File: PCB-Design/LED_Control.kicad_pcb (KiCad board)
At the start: 2 copper layers, 60 x 80 mm, 28 parts, among them J1 5V 5A Power, J2 TO WS2812B LED STRIP, J3 Sound Sensor, SW1 SW_Push_Dual

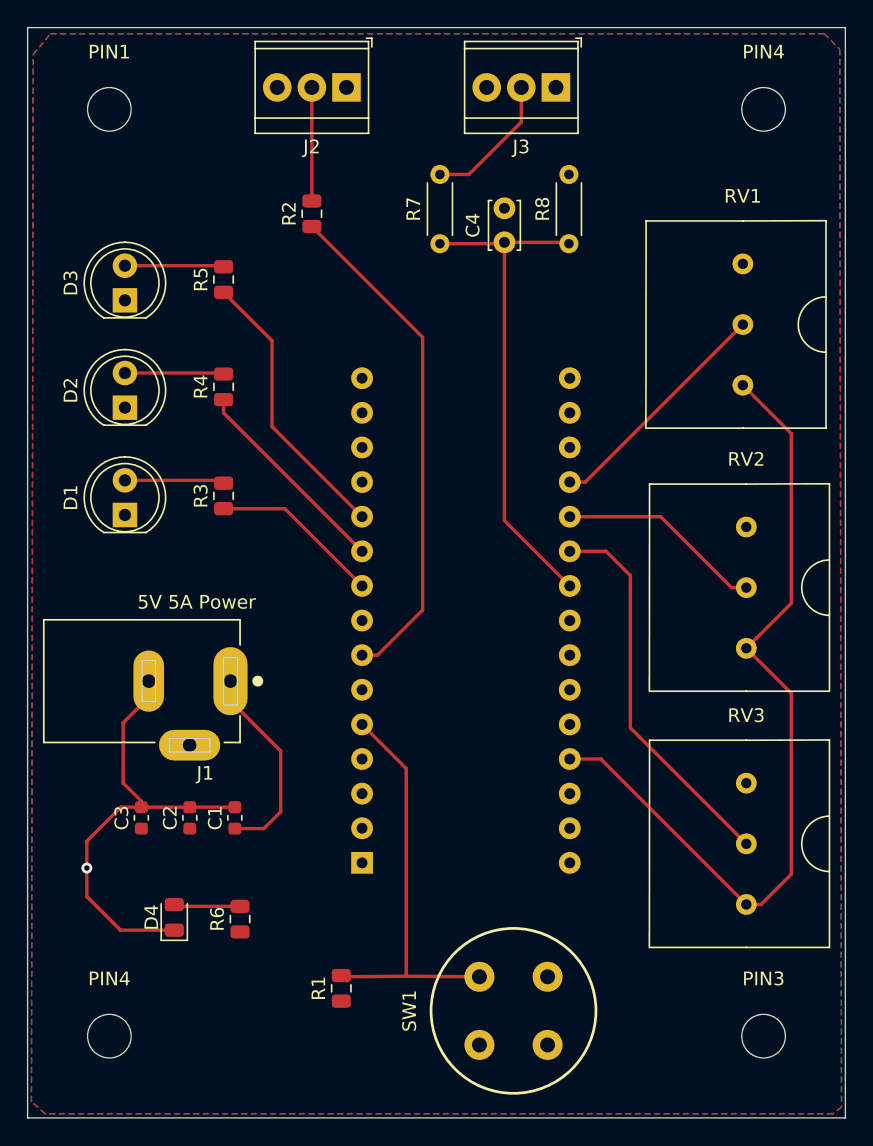
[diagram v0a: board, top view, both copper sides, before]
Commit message: final submitted build files
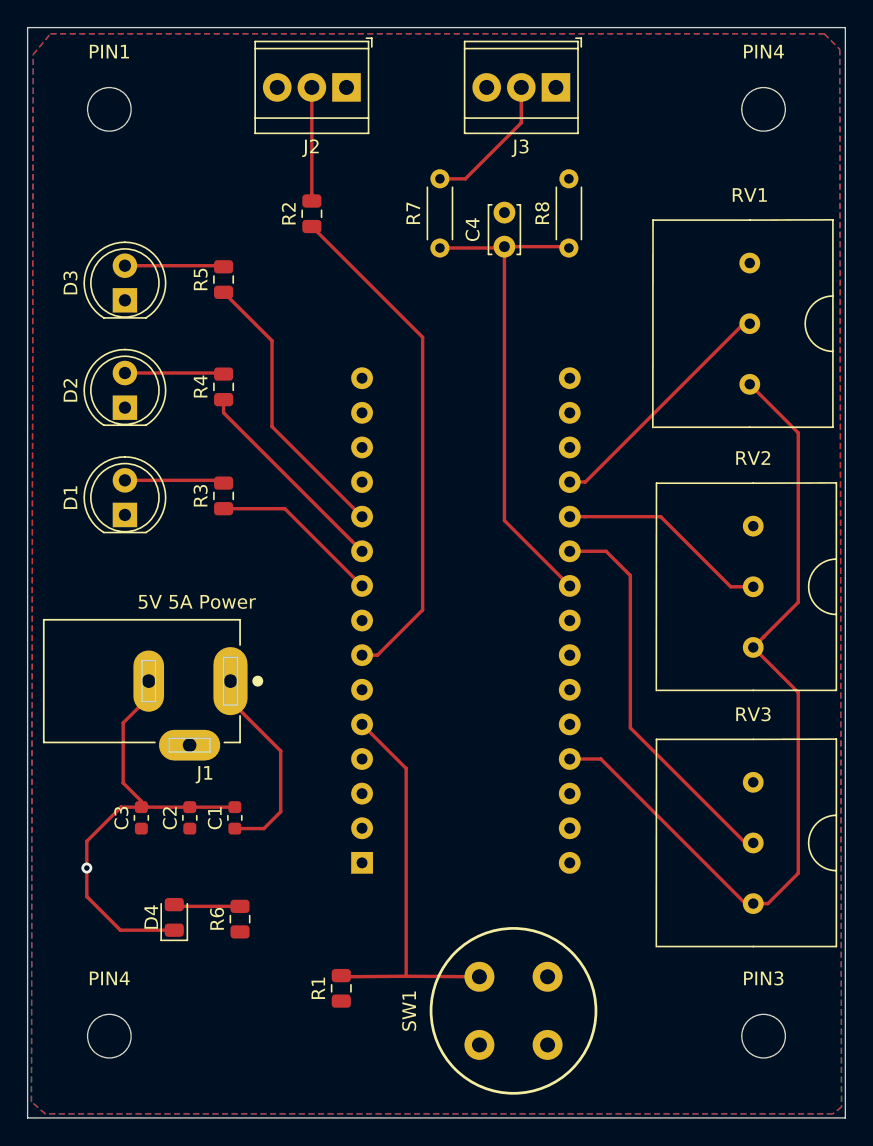
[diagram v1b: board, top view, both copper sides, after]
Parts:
- R6: value 100 -> 200
- moved RV1 0.51 mm to (158.0, 81.7)
- moved RV2 0.51 mm to (158.2, 101.0)
- moved RV3 0.51 mm to (158.2, 119.8)
- moved C4 0.32 mm to (140.0, 76.1)
- moved R7 0.32 mm to (135.3, 76.2)
- moved R8 0.32 mm to (144.7, 76.2)
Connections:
- J3 pad 1: GND -> VCC
- J3 pad 3: VCC -> GND
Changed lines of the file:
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@@
     (47 F.CrtYd user)
     (48 B.Fab user)
-    (49 F.Fab user hide)
+    (49 F.Fab user)
   )
   (setup
@@
   )
   (module Resistor_THT:R_Axial_DIN0204_L3.6mm_D1.6mm_P5.08mm_Horizontal (layer F.Cu)
-    (at 144.7165 75.8555 90)
+    (at 144.7165 76.173 90)
     (descr "Resistor, Axial_DIN0204 series, Axial, Horizontal, pin pitch=5.08mm, 0.167W, length*diameter=3.6*1.6mm^2, http://cdn-reichelt.de/documents/datenblatt/B400/1_4W%23YAG.pdf")
     (tags "Resistor Axial_DIN0204 series Axial Horizontal pin pitch 5.08mm 0.167W length 3.6mm diameter 1.6mm")
@@
     (fp_circle (center 0 0) (end 1.1 0) (layer F.Fab) (width 0.1))
     (pad 3 thru_hole circle (at 5.08 0 180) (size 2.1 2.1) (drill 1.1) (layers *.Cu *.Mask)
-      (net 27 VCC))
+      (net 25 GND))
     (pad 2 thru_hole circle (at 2.54 0 180) (size 2.1 2.1) (drill 1.1) (layers *.Cu *.Mask)
       (net 37 /SS_DATA_OUT))
     (pad 1 thru_hole rect (at 0 0 180) (size 2.1 2.1) (drill 1.1) (layers *.Cu *.Mask)
-      (net 25 GND))
+      (net 27 VCC))
     (model ${KISYS3DMOD}/TerminalBlock_TE-Connectivity.3dshapes/TerminalBlock_TE_282834-3_1x03_P2.54mm_Horizontal.wrl
       (at (xyz 0 0 0))
@@
   )
   (module Resistor_THT:R_Axial_DIN0204_L3.6mm_D1.6mm_P5.08mm_Horizontal (layer F.Cu)
-    (at 135.255 75.8555 90)
+    (at 135.255 76.173 90)
     (descr "Resistor, Axial_DIN0204 series, Axial, Horizontal, pin pitch=5.08mm, 0.167W, length*diameter=3.6*1.6mm^2, http://cdn-reichelt.de/documents/datenblatt/B400/1_4W%23YAG.pdf")
     (tags "Resistor Axial_DIN0204 series Axial Horizontal pin pitch 5.08mm 0.167W length 3.6mm diameter 1.6mm")
@@
   )
   (module Capacitor_THT:C_Disc_D3.4mm_W2.1mm_P2.50mm (layer F.Cu)
-    (at 139.98575 75.7555 90)
+    (at 139.98575 76.073 90)
     (descr "C, Disc series, Radial, pin pitch=2.50mm, , diameter*width=3.4*2.1mm^2, Capacitor, http://www.vishay.com/docs/45233/krseries.pdf")
     (tags "C Disc series Radial pin pitch 2.50mm  diameter 3.4mm width 2.1mm Capacitor")
@@
       (effects (font (size 1 1) (thickness 0.15)))
     )
-    (fp_text value 100 (at 0 1.65 90) (layer F.Fab)
+    (fp_text value 200 (at 0 1.65 90) (layer F.Fab)
       (effects (font (size 1 1) (thickness 0.15)))
     )
@@
   )
   (module "Custom Footprint:Potentiometer_4mm_Pitch" (layer F.Cu)
-    (at 157.48 81.788)
+    (at 157.988 81.7245)
     (fp_text reference RV1 (at 0 -9.406) (layer F.SilkS)
       (effects (font (size 1 1) (thickness 0.15)))
@@
   )
   (module "Custom Footprint:Potentiometer_4mm_Pitch" (layer F.Cu)
-    (at 157.734 101.092)
+    (at 158.242 101.0285)
     (fp_text reference RV2 (at 0 -9.406) (layer F.SilkS)
       (effects (font (size 1 1) (thickness 0.15)))
@@
   )
   (module "Custom Footprint:Potentiometer_4mm_Pitch" (layer F.Cu)
-    (at 157.734 119.888)
+    (at 158.242 119.8245)
     (fp_text reference RV3 (at 0 -9.406) (layer F.SilkS)
       (effects (font (size 1 1) (thickness 0.15)))
@@
   (segment (start 145.91137 95.885) (end 144.78 95.885) (width 0.25) (layer F.Cu) (net 8))
   (segment (start 151.44937 95.885) (end 145.91137 95.885) (width 0.25) (layer F.Cu) (net 8))
-  (segment (start 156.65637 101.092) (end 151.44937 95.885) (width 0.25) (layer F.Cu) (net 8))
-  (segment (start 157.734 101.092) (end 156.65637 101.092) (width 0.25) (layer F.Cu) (net 8))
+  (segment (start 158.242 101.0285) (end 156.59287 101.0285) (width 0.25) (layer F.Cu) (net 8))
+  (segment (start 156.59287 101.0285) (end 151.44937 95.885) (width 0.25) (layer F.Cu) (net 8))
   (segment (start 128.1045 129.6435) (end 128.016 129.555) (width 0.25) (layer F.Cu) (net 9))
   (segment (start 132.7785 114.3635) (end 132.7785 129.6035) (width 0.25) (layer F.Cu) (net 9))
@@
   (segment (start 147.061 113.665) (end 144.78 113.665) (width 0.25) (layer F.Cu) (net 21))
   (segment (start 157.734 124.338) (end 147.061 113.665) (width 0.25) (layer F.Cu) (net 21))
-  (segment (start 158.81163 124.338) (end 161.036 122.11363) (width 0.25) (layer F.Cu) (net 21))
-  (segment (start 157.734 124.338) (end 158.81163 124.338) (width 0.25) (layer F.Cu) (net 21))
-  (segment (start 161.036 108.844) (end 157.734 105.542) (width 0.25) (layer F.Cu) (net 21))
-  (segment (start 161.036 122.11363) (end 161.036 108.844) (width 0.25) (layer F.Cu) (net 21))
-  (segment (start 158.495999 104.780001) (end 158.495999 104.775001) (width 0.25) (layer F.Cu) (net 21))
-  (segment (start 157.734 105.542) (end 158.495999 104.780001) (width 0.25) (layer F.Cu) (net 21))
-  (segment (start 158.495999 104.775001) (end 161.036 102.235) (width 0.25) (layer F.Cu) (net 21))
-  (segment (start 161.036 89.794) (end 157.48 86.238) (width 0.25) (layer F.Cu) (net 21))
-  (segment (start 161.036 102.235) (end 161.036 89.794) (width 0.25) (layer F.Cu) (net 21))
+  (segment (start 159.31963 124.2745) (end 161.544 122.05013) (width 0.25) (layer F.Cu) (net 21))
+  (segment (start 158.242 124.2745) (end 159.31963 124.2745) (width 0.25) (layer F.Cu) (net 21))
+  (segment (start 161.544 108.7805) (end 158.242 105.4785) (width 0.25) (layer F.Cu) (net 21))
+  (segment (start 161.544 122.05013) (end 161.544 108.7805) (width 0.25) (layer F.Cu) (net 21))
+  (segment (start 159.003999 104.716501) (end 159.003999 104.711501) (width 0.25) (layer F.Cu) (net 21))
+  (segment (start 158.242 105.4785) (end 159.003999 104.716501) (width 0.25) (layer F.Cu) (net 21))
+  (segment (start 159.003999 104.711501) (end 161.544 102.1715) (width 0.25) (layer F.Cu) (net 21))
+  (segment (start 161.544 89.7305) (end 157.988 86.1745) (width 0.25) (layer F.Cu) (net 21))
+  (segment (start 161.544 102.1715) (end 161.544 89.7305) (width 0.25) (layer F.Cu) (net 21))
   (segment (start 113.8225 117.1955) (end 116.9035 117.1955) (width 0.25) (layer F.Cu) (net 25))
   (segment (start 113.3475 117.1955) (end 113.8225 117.1955) (width 0.25) (layer F.Cu) (net 25))
@@
   (segment (start 123.571 113.073416) (end 120.522644 110.02506) (width 0.25) (layer F.Cu) (net 27))
   (segment (start 123.571 117.5385) (end 123.571 113.073416) (width 0.25) (layer F.Cu) (net 27))
-  (segment (start 139.88575 75.8555) (end 139.98575 75.7555) (width 0.25) (layer F.Cu) (net 30))
-  (segment (start 135.255 75.8555) (end 139.88575 75.8555) (width 0.25) (layer F.Cu) (net 30))
-  (segment (start 144.6165 75.7555) (end 144.7165 75.8555) (width 0.25) (layer F.Cu) (net 30))
-  (segment (start 139.98575 75.7555) (end 144.6165 75.7555) (width 0.25) (layer F.Cu) (net 30))
+  (segment (start 139.88575 76.173) (end 139.98575 76.073) (width 0.25) (layer F.Cu) (net 30))
+  (segment (start 135.255 76.173) (end 139.88575 76.173) (width 0.25) (layer F.Cu) (net 30))
+  (segment (start 144.6165 76.073) (end 144.7165 76.173) (width 0.25) (layer F.Cu) (net 30))
+  (segment (start 139.98575 76.073) (end 144.6165 76.073) (width 0.25) (layer F.Cu) (net 30))
   (segment (start 139.98575 96.17075) (end 144.78 100.965) (width 0.25) (layer F.Cu) (net 30))
-  (segment (start 139.98575 75.7555) (end 139.98575 96.17075) (width 0.25) (layer F.Cu) (net 30))
+  (segment (start 139.98575 76.073) (end 139.98575 96.17075) (width 0.25) (layer F.Cu) (net 30))
   (segment (start 119.253 93.1695) (end 119.507 93.4235) (width 0.25) (layer F.Cu) (net 31))
   (segment (start 119.1745 93.218) (end 119.38 93.4235) (width 0.25) (layer F.Cu) (net 31))
@@
   (segment (start 125.857 72.235) (end 125.857 64.389) (width 0.25) (layer F.Cu) (net 36))
   (segment (start 125.857 72.7225) (end 125.857 72.235) (width 0.25) (layer F.Cu) (net 36))
-  (segment (start 135.255 70.7755) (end 137.3775 70.7755) (width 0.25) (layer F.Cu) (net 37))
-  (segment (start 141.224 66.929) (end 141.224 64.389) (width 0.25) (layer F.Cu) (net 37))
-  (segment (start 137.3775 70.7755) (end 141.224 66.929) (width 0.25) (layer F.Cu) (net 37))
+  (segment (start 141.224 66.9925) (end 141.224 64.389) (width 0.25) (layer F.Cu) (net 37))
+  (segment (start 137.1235 71.093) (end 141.224 66.9925) (width 0.25) (layer F.Cu) (net 37))
+  (segment (start 135.255 71.093) (end 137.1235 71.093) (width 0.25) (layer F.Cu) (net 37))
   (zone (net 27) (net_name VCC) (layer F.Cu) (hatch edge 0.508)
     (connect_pads (clearance 0.508))
